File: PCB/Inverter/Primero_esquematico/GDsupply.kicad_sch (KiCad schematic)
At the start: 44 parts, among them T1 750317595, U10 UCC21750QDWRQ1, U40 LM25180QNGURQ1

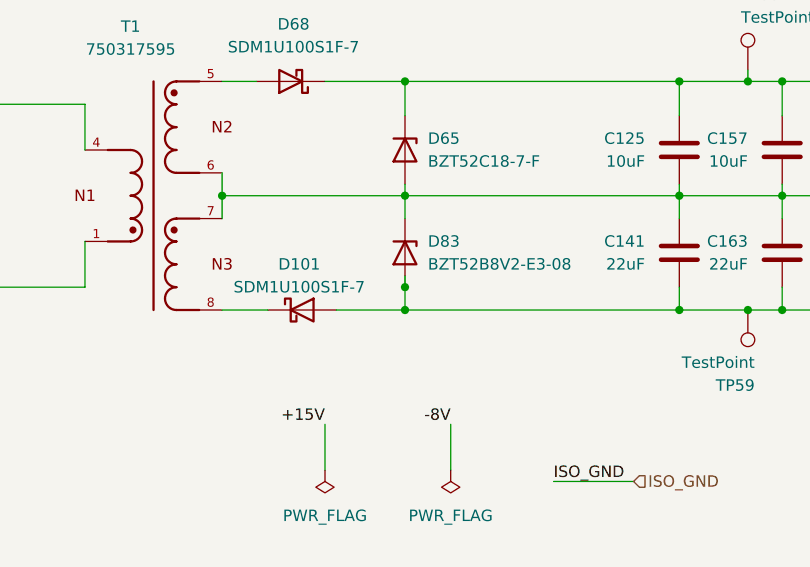
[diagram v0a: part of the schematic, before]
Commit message: Sigo con la placa padre
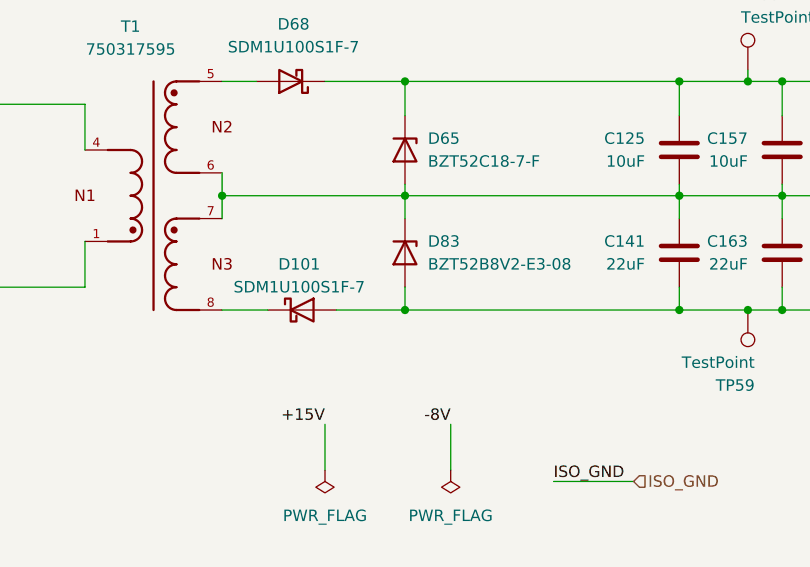
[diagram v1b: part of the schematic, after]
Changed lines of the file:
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@@
-	)
-	(junction
-		(at 209.55 59.69)
-		(diameter 0)
-		(color 0 0 0 0)
 	)
 	(junction
@@
 		)
 		(stroke
-			(width 0)
-			(type default)
-		)
-	)
-	(wire
-		(pts
-			(xy 209.55 58.42) (xy 209.55 59.69)
-		)
-		(stroke

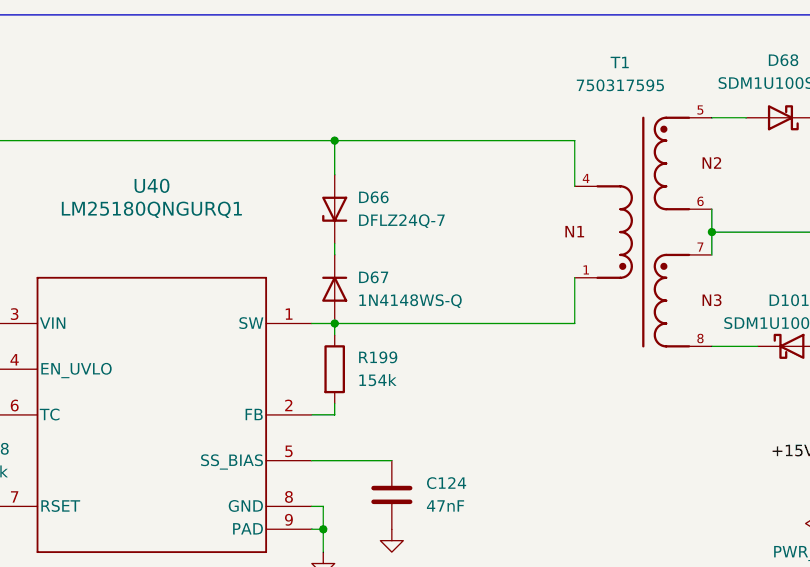
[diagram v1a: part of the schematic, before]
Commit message: Casi todo padre
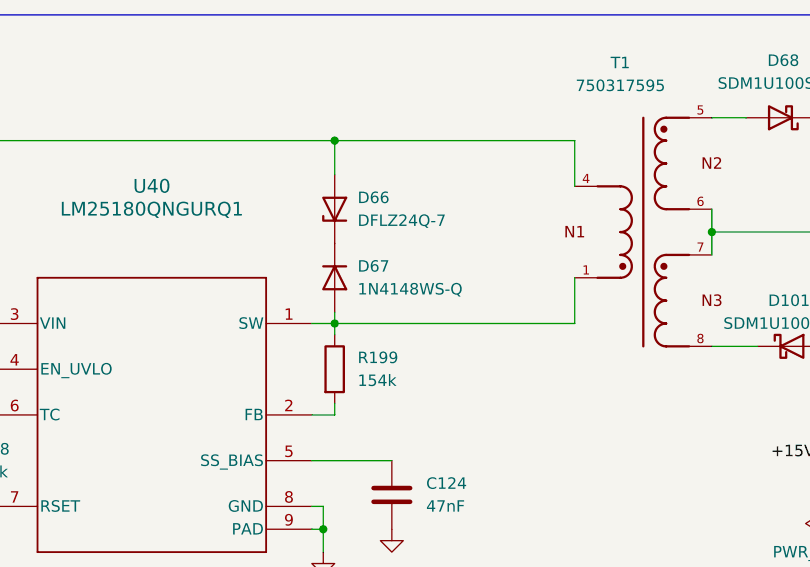
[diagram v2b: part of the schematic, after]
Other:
- moved on the sheet: D67
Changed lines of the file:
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@@
 	(wire
 		(pts
+			(xy 147.32 58.42) (xy 147.32 59.69)
+		)
+		(stroke
+			(width 0)
+			(type default)
+		)
+	)
+	(wire
+		(pts
 			(xy 208.28 111.76) (xy 234.95 111.76)
 		)
@@
 	(wire
 		(pts
-			(xy 147.32 50.8) (xy 147.32 52.07)
-		)
-		(stroke
-			(width 0)
-			(type default)
-		)
-	)
-	(wire
-		(pts
 			(xy 127 129.54) (xy 134.62 129.54)
 		)
@@
 	(symbol
 		(lib_id "Device:D")
-		(at 147.32 55.88 270)
+		(at 147.32 54.61 270)
 		(unit 1)
 		(body_style 1)
@@
 		(fields_autoplaced yes)
 		(property "Reference" "D67"
-			(at 149.86 54.6099 90)
+			(at 149.86 53.3399 90)
 			(show_name no)
 			(do_not_autoplace no)
@@
 		)
 		(property "Value" "1N4148WS-Q"
-			(at 149.86 57.1499 90)
+			(at 149.86 55.8799 90)
 			(show_name no)
 			(do_not_autoplace no)
@@
 		)
 		(property "Footprint" "Diode_SMD:D_SOD-323F"
-			(at 147.32 55.88 0)
+			(at 147.32 54.61 0)
 			(hide yes)
 			(show_name no)
@@
 		)
 		(property "Datasheet" "https://diotec.com/request/datasheet/1n4148ws.pdf"
-			(at 147.32 55.88 0)
+			(at 147.32 54.61 0)
 			(hide yes)
 			(show_name no)
@@
 		)
 		(property "Description" "Diode"
-			(at 147.32 55.88 0)
+			(at 147.32 54.61 0)
 			(hide yes)
 			(show_name no)
@@
 		)
 		(property "Sim.Device" "D"
-			(at 147.32 55.88 0)
+			(at 147.32 54.61 0)
 			(hide yes)
 			(show_name no)
@@
 		)
 		(property "Sim.Pins" "1=K 2=A"
-			(at 147.32 55.88 0)
+			(at 147.32 54.61 0)
 			(hide yes)
 			(show_name no)
@@
 		)
 		(property "Compra" "https://www.digikey.com/en/products/detail/diotec-semiconductor/1N4148WS-Q/22522880?s=N4IgTCBcDaICwA4DsCC0BGAcndiDqAyqgIoDCAKqpgCIgC6AvkA"
-			(at 147.32 55.88 0)
+			(at 147.32 54.61 0)
 			(hide yes)
 			(show_name no)
